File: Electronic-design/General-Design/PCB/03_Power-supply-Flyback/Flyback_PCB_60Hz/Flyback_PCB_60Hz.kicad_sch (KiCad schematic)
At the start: 53 parts, among them IC4 UCC38C43DGKR, J1 4300.0104, J6 Conn_01x02, Q1 NMOS, Q2 PNP, Q3 NPN, T2 Transformer_1P_2S, U1 4N35, U2 TL431LP

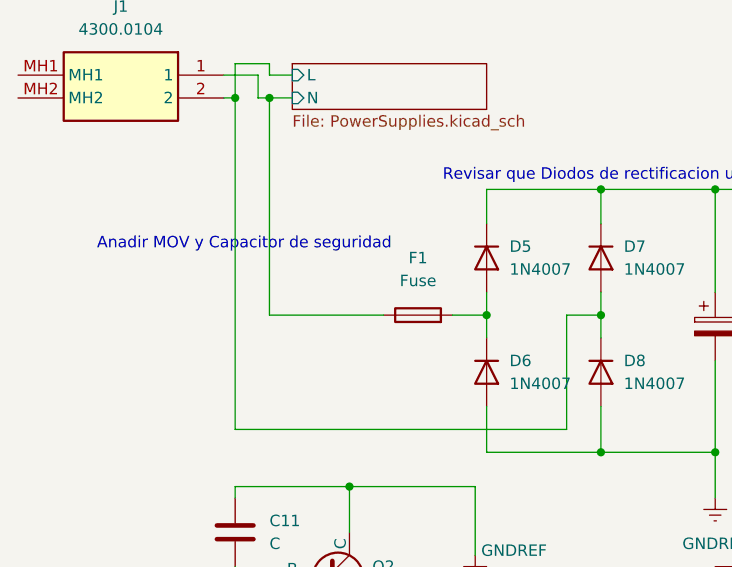
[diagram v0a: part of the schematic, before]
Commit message: MOV
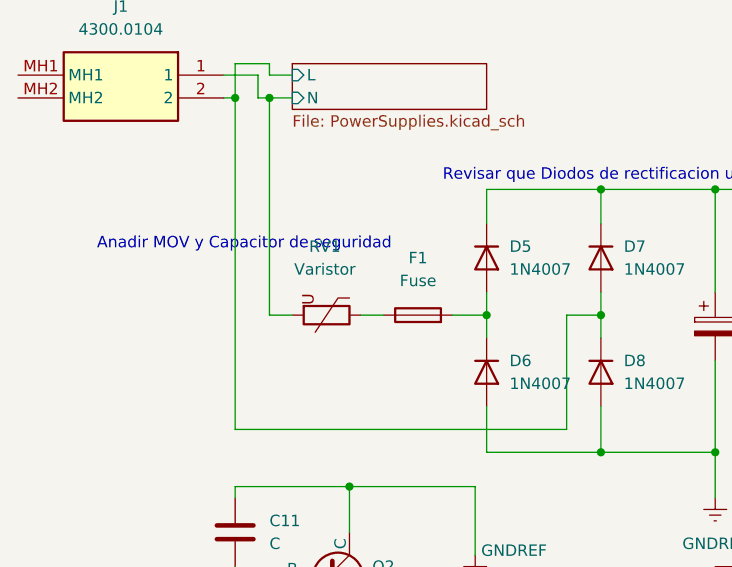
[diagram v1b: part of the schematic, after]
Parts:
- added RV1: Varistor, symbol Device:Varistor
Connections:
- net Supplies/N: now also RV1.2; no longer F1.1
- new net: F1.1, RV1.1
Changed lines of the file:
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@@
 	(wire
 		(pts
+			(xy 50.8 48.26) (xy 53.34 48.26)
+		)
+		(stroke
+			(width 0)
+			(type default)
+		)
+	)
+	(wire
+		(pts
 			(xy 168.91 24.13) (xy 168.91 41.91)
 		)
@@
 	(wire
 		(pts
-			(xy 40.64 48.26) (xy 53.34 48.26)
-		)
-		(stroke
-			(width 0)
-			(type default)
-		)
-	)
-	(wire
-		(pts
 			(xy 168.91 111.76) (xy 168.91 110.49)
 		)
@@
 	(wire
 		(pts
+			(xy 40.64 48.26) (xy 43.18 48.26)
+		)
+		(stroke
+			(width 0)
+			(type default)
+		)
+	)
+	(wire
+		(pts
 			(xy 227.33 161.29) (xy 227.33 160.02)
 		)
@@
 					(unit 1)
 				)
+			)
+		)
+	)
+	(symbol
+		(lib_id "Device:Varistor")
+		(at 46.99 48.26 270)
+		(unit 1)
+		(exclude_from_sim no)
+		(in_bom yes)
+		(on_board yes)
+		(dnp no)
+		(fields_autoplaced yes)
+		(property "Reference" "RV1"
+			(at 46.7966 40.64 90)
+			(effects
+				(font
+					(size 1.27 1.27)
+				)
+			)
+		)
+		(property "Value" "Varistor"
+			(at 46.7966 43.18 90)
+			(effects
+				(font
+					(size 1.27 1.27)
+				)
+			)
+		)
+		(property "Footprint" ""
+			(at 46.99 46.482 90)
+			(effects
+				(font
+					(size 1.27 1.27)
+				)
+				(hide yes)
+			)
+		)
+		(property "Datasheet" "~"
+			(at 46.99 48.26 0)
+			(effects
+				(font
+					(size 1.27 1.27)
+				)
+				(hide yes)
+			)
+		)
+		(property "Description" "Voltage dependent resistor"
+			(at 46.99 48.26 0)
+			(effects
+				(font
+					(size 1.27 1.27)
+				)
+				(hide yes)
+			)
+		)
+		(property "Sim.Name" "kicad_builtin_varistor"
+			(at 46.99 48.26 0)
+			(effects
+				(font
+					(size 1.27 1.27)
+				)
+				(hide yes)
+			)
+		)
+		(property "Sim.Device" "SUBCKT"
+			(at 46.99 48.26 0)
+			(effects
+				(font
+					(size 1.27 1.27)
+				)
+				(hide yes)
+			)
+		)
+		(property "Sim.Pins" "1=A 2=B"
+			(at 46.99 48.26 0)
+			(effects
+				(font
+					(size 1.27 1.27)
+				)
+				(hide yes)
+			)
+		)
+		(property "Sim.Params" "threshold=1k"
+			(at 46.99 48.26 0)
+			(effects
+				(font
+					(size 1.27 1.27)
+				)
+				(hide yes)
+			)
+		)
+		(property "Sim.Library" "${KICAD7_SYMBOL_DIR}/Simulation_SPICE.sp"
+			(at 46.99 48.26 0)
+			(effects
+				(font
+					(size 1.27 1.27)
+				)
+				(hide yes)
+			)
+		)
+		(pin "1"
+		)
+		(pin "2"
+		)
+		(instances
+			(project ""
+				(path "/e667b3b5-58bf-48ce-ba71-7e90a3c6a4c9"
+					(reference "RV1")
+					(unit 1)
+				)
